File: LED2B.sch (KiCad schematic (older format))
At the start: 17 parts

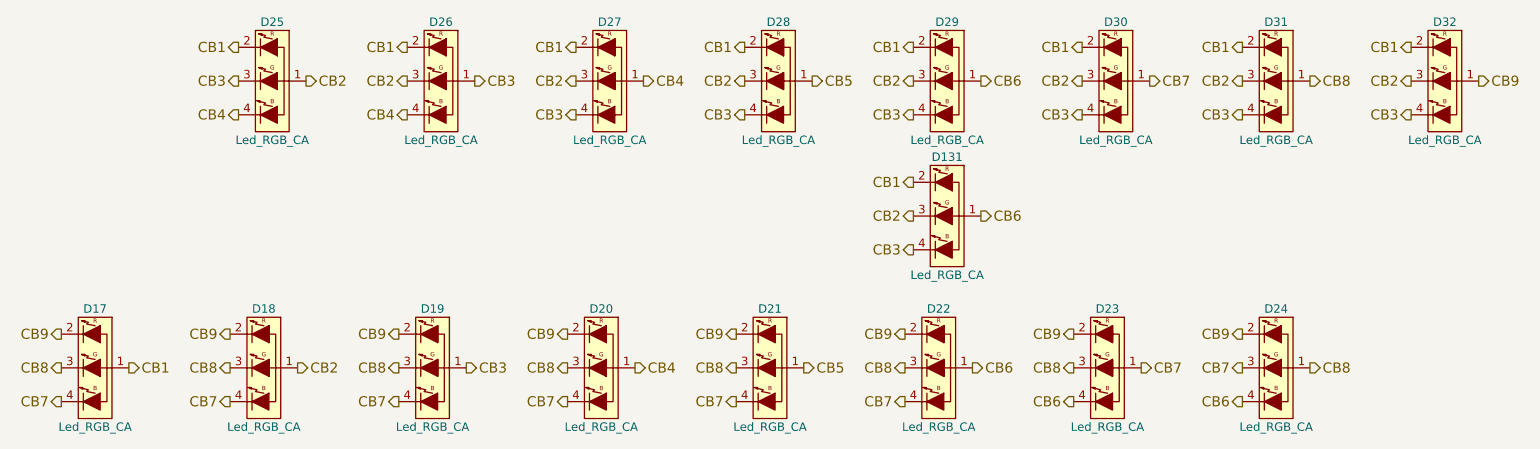
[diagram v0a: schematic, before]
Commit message: Did some visual cleanup.
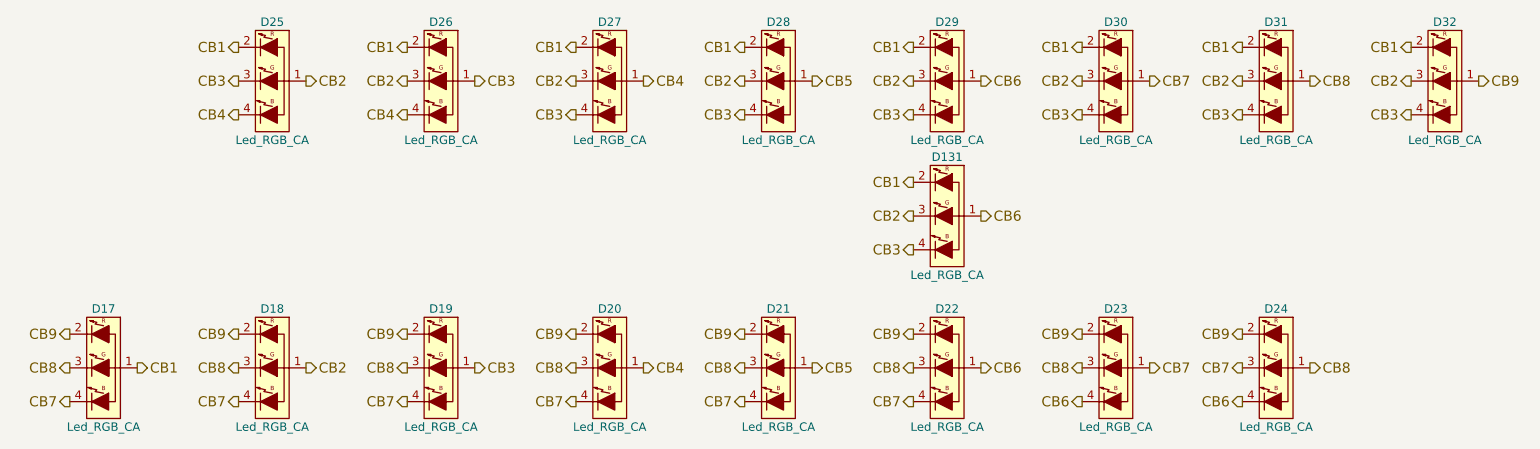
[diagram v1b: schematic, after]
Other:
- moved on the sheet: D17, D18, D19, D20, D21, D22, D23
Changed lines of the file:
@@
 $Descr A4 11693 8268
 encoding utf-8
-Sheet 3 6
+Sheet 2 6
 Title ""
 Date ""
@@
 Text HLabel 9750 1550 0    60   Output ~ 0
 CB1
-Text HLabel 2150 3450 2    60   Output ~ 0
-CB1
-Text HLabel 1750 3650 0    60   Output ~ 0
-CB7
-Text HLabel 1750 3450 0    60   Output ~ 0
-CB8
-Text HLabel 1750 3250 0    60   Output ~ 0
-CB9
-Text HLabel 2750 3650 0    60   Output ~ 0
-CB7
-Text HLabel 2750 3450 0    60   Output ~ 0
-CB8
-Text HLabel 2750 3250 0    60   Output ~ 0
-CB9
-Text HLabel 3150 3450 2    60   Output ~ 0
-CB2
-Text HLabel 3750 3650 0    60   Output ~ 0
-CB7
-Text HLabel 3750 3450 0    60   Output ~ 0
-CB8
-Text HLabel 3750 3250 0    60   Output ~ 0
-CB9
-Text HLabel 4150 3450 2    60   Output ~ 0
-CB3
-Text HLabel 4750 3650 0    60   Output ~ 0
-CB7
-Text HLabel 4750 3450 0    60   Output ~ 0
-CB8
-Text HLabel 4750 3250 0    60   Output ~ 0
-CB9
-Text HLabel 5150 3450 2    60   Output ~ 0
+Text HLabel 2200 3450 2    60   Output ~ 0
+CB1
+Text HLabel 1800 3650 0    60   Output ~ 0
+CB7
+Text HLabel 1800 3450 0    60   Output ~ 0
+CB8
+Text HLabel 1800 3250 0    60   Output ~ 0
+CB9
+Text HLabel 2800 3650 0    60   Output ~ 0
+CB7
+Text HLabel 2800 3450 0    60   Output ~ 0
+CB8
+Text HLabel 2800 3250 0    60   Output ~ 0
+CB9
+Text HLabel 3200 3450 2    60   Output ~ 0
+CB2
+Text HLabel 3800 3650 0    60   Output ~ 0
+CB7
+Text HLabel 3800 3450 0    60   Output ~ 0
+CB8
+Text HLabel 3800 3250 0    60   Output ~ 0
+CB9
+Text HLabel 4200 3450 2    60   Output ~ 0
+CB3
+Text HLabel 4800 3650 0    60   Output ~ 0
+CB7
+Text HLabel 4800 3450 0    60   Output ~ 0
+CB8
+Text HLabel 4800 3250 0    60   Output ~ 0
+CB9
+Text HLabel 5200 3450 2    60   Output ~ 0
 CB4
-Text HLabel 5750 3650 0    60   Output ~ 0
-CB7
-Text HLabel 5750 3450 0    60   Output ~ 0
-CB8
-Text HLabel 5750 3250 0    60   Output ~ 0
-CB9
-Text HLabel 6150 3450 2    60   Output ~ 0
+Text HLabel 5800 3650 0    60   Output ~ 0
+CB7
+Text HLabel 5800 3450 0    60   Output ~ 0
+CB8
+Text HLabel 5800 3250 0    60   Output ~ 0
+CB9
+Text HLabel 6200 3450 2    60   Output ~ 0
 CB5
-Text HLabel 6750 3650 0    60   Output ~ 0
-CB7
-Text HLabel 6750 3450 0    60   Output ~ 0
-CB8
-Text HLabel 6750 3250 0    60   Output ~ 0
-CB9
-Text HLabel 7150 3450 2    60   Output ~ 0
+Text HLabel 6800 3650 0    60   Output ~ 0
+CB7
+Text HLabel 6800 3450 0    60   Output ~ 0
+CB8
+Text HLabel 6800 3250 0    60   Output ~ 0
+CB9
+Text HLabel 7200 3450 2    60   Output ~ 0
 CB6
-Text HLabel 8150 3450 2    60   Output ~ 0
-CB7
-Text HLabel 7750 3450 0    60   Output ~ 0
-CB8
-Text HLabel 7750 3250 0    60   Output ~ 0
-CB9
-Text HLabel 7750 3650 0    60   Output ~ 0
+Text HLabel 8200 3450 2    60   Output ~ 0
+CB7
+Text HLabel 7800 3450 0    60   Output ~ 0
+CB8
+Text HLabel 7800 3250 0    60   Output ~ 0
+CB9
+Text HLabel 7800 3650 0    60   Output ~ 0
 CB6
 Text HLabel 8750 3250 0    60   Output ~ 0
@@
 L Led_RGB_CA D17
 U 1 1 56C5D501
-P 1950 3450
-F 0 "D17" H 1950 3800 50  0000 C CNN
-F 1 "Led_RGB_CA" H 1950 3100 50  0000 C CNN
-F 2 "mx2a:RGB" H 1905 3400 50  0001 C CNN
-F 3 "" H 1905 3400 50  0000 C CNN
-	1    1950 3450
+P 2000 3450
+F 0 "D17" H 2000 3800 50  0000 C CNN
+F 1 "Led_RGB_CA" H 2000 3100 50  0000 C CNN
+F 2 "mx2a:RGB" H 1955 3400 50  0001 C CNN
+F 3 "" H 1955 3400 50  0000 C CNN
+	1    2000 3450
 	1    0    0    -1
 $EndComp
@@
 L Led_RGB_CA D18
 U 1 1 56C5DE77
-P 2950 3450
-F 0 "D18" H 2950 3800 50  0000 C CNN
-F 1 "Led_RGB_CA" H 2950 3100 50  0000 C CNN
-F 2 "mx2a:RGB" H 2905 3400 50  0001 C CNN
-F 3 "" H 2905 3400 50  0000 C CNN
-	1    2950 3450
+P 3000 3450
+F 0 "D18" H 3000 3800 50  0000 C CNN
+F 1 "Led_RGB_CA" H 3000 3100 50  0000 C CNN
+F 2 "mx2a:RGB" H 2955 3400 50  0001 C CNN
+F 3 "" H 2955 3400 50  0000 C CNN
+	1    3000 3450
 	1    0    0    -1
 $EndComp
@@
 L Led_RGB_CA D19
 U 1 1 56C5DEC1
-P 3950 3450
-F 0 "D19" H 3950 3800 50  0000 C CNN
-F 1 "Led_RGB_CA" H 3950 3100 50  0000 C CNN
-F 2 "mx2a:RGB" H 3905 3400 50  0001 C CNN
-F 3 "" H 3905 3400 50  0000 C CNN
-	1    3950 3450
+P 4000 3450
+F 0 "D19" H 4000 3800 50  0000 C CNN
+F 1 "Led_RGB_CA" H 4000 3100 50  0000 C CNN
+F 2 "mx2a:RGB" H 3955 3400 50  0001 C CNN
+F 3 "" H 3955 3400 50  0000 C CNN
+	1    4000 3450
 	1    0    0    -1
 $EndComp
@@
 L Led_RGB_CA D20
 U 1 1 56C5DF12
-P 4950 3450
-F 0 "D20" H 4950 3800 50  0000 C CNN
-F 1 "Led_RGB_CA" H 4950 3100 50  0000 C CNN
-F 2 "mx2a:RGB" H 4905 3400 50  0001 C CNN
-F 3 "" H 4905 3400 50  0000 C CNN
-	1    4950 3450
+P 5000 3450
+F 0 "D20" H 5000 3800 50  0000 C CNN
+F 1 "Led_RGB_CA" H 5000 3100 50  0000 C CNN
+F 2 "mx2a:RGB" H 4955 3400 50  0001 C CNN
+F 3 "" H 4955 3400 50  0000 C CNN
+	1    5000 3450
 	1    0    0    -1
 $EndComp
@@
 L Led_RGB_CA D21
 U 1 1 56C5E004
-P 5950 3450
-F 0 "D21" H 5950 3800 50  0000 C CNN
-F 1 "Led_RGB_CA" H 5950 3100 50  0000 C CNN
-F 2 "mx2a:RGB" H 5905 3400 50  0001 C CNN
-F 3 "" H 5905 3400 50  0000 C CNN
-	1    5950 3450
+P 6000 3450
+F 0 "D21" H 6000 3800 50  0000 C CNN
+F 1 "Led_RGB_CA" H 6000 3100 50  0000 C CNN
+F 2 "mx2a:RGB" H 5955 3400 50  0001 C CNN
+F 3 "" H 5955 3400 50  0000 C CNN
+	1    6000 3450
 	1    0    0    -1
 $EndComp
@@
 L Led_RGB_CA D22
 U 1 1 56C5E0ED
-P 6950 3450
-F 0 "D22" H 6950 3800 50  0000 C CNN
-F 1 "Led_RGB_CA" H 6950 3100 50  0000 C CNN
-F 2 "mx2a:RGB" H 6905 3400 50  0001 C CNN
-F 3 "" H 6905 3400 50  0000 C CNN
-	1    6950 3450
+P 7000 3450
+F 0 "D22" H 7000 3800 50  0000 C CNN
+F 1 "Led_RGB_CA" H 7000 3100 50  0000 C CNN
+F 2 "mx2a:RGB" H 6955 3400 50  0001 C CNN
+F 3 "" H 6955 3400 50  0000 C CNN
+	1    7000 3450
 	1    0    0    -1
 $EndComp
@@
 L Led_RGB_CA D23
 U 1 1 56C5E285
-P 7950 3450
-F 0 "D23" H 7950 3800 50  0000 C CNN
-F 1 "Led_RGB_CA" H 7950 3100 50  0000 C CNN
-F 2 "mx2a:RGB" H 7905 3400 50  0001 C CNN
-F 3 "" H 7905 3400 50  0000 C CNN
-	1    7950 3450
-	1    0    0    -1
-$EndComp
+P 8000 3450
+F 0 "D23" H 8000 3800 50  0000 C CNN
+F 1 "Led_RGB_CA" H 8000 3100 50  0000 C CNN
+F 2 "mx2a:RGB" H 7955 3400 50  0001 C CNN
+F 3 "" H 7955 3400 50  0000 C CNN
+	1    8000 3450
+	1    0    0    -1
+$EndComp

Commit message: Switched to a different USB Port and 100uF Cap
also added a USB-Debug Header and did some cleanup
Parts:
- D131, D17, D18, D19, D20, D21, D22, D23, D24, D25, D26, D27, D28, D29, D30, D31, D32: footprint mx2a:RGB -> libs.pretty:RGB
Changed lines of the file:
@@
 U 1 1 56C58153
 P 3000 1750
+AR Path="/56C58153" Ref="D25"  Part="1"
+AR Path="/572AC680/56C58153" Ref="D25"  Part="1"
 F 0 "D25" H 3000 2100 50  0000 C CNN
 F 1 "Led_RGB_CA" H 3000 1400 50  0000 C CNN
-F 2 "mx2a:RGB" H 2955 1700 50  0001 C CNN
+F 2 "libs.pretty:RGB" H 2955 1700 50  0001 C CNN
 F 3 "" H 2955 1700 50  0000 C CNN
 	1    3000 1750
@@
 U 1 1 56C58187
 P 4000 1750
+AR Path="/56C58187" Ref="D26"  Part="1"
+AR Path="/572AC680/56C58187" Ref="D26"  Part="1"
 F 0 "D26" H 4000 2100 50  0000 C CNN
 F 1 "Led_RGB_CA" H 4000 1400 50  0000 C CNN
-F 2 "mx2a:RGB" H 3955 1700 50  0001 C CNN
+F 2 "libs.pretty:RGB" H 3955 1700 50  0001 C CNN
 F 3 "" H 3955 1700 50  0000 C CNN
 	1    4000 1750
@@
 U 1 1 56C581B9
 P 5000 1750
+AR Path="/56C581B9" Ref="D27"  Part="1"
+AR Path="/572AC680/56C581B9" Ref="D27"  Part="1"
 F 0 "D27" H 5000 2100 50  0000 C CNN
 F 1 "Led_RGB_CA" H 5000 1400 50  0000 C CNN
-F 2 "mx2a:RGB" H 4955 1700 50  0001 C CNN
+F 2 "libs.pretty:RGB" H 4955 1700 50  0001 C CNN
 F 3 "" H 4955 1700 50  0000 C CNN
 	1    5000 1750
@@
 U 1 1 56C5823E
 P 6000 1750
+AR Path="/56C5823E" Ref="D28"  Part="1"
+AR Path="/572AC680/56C5823E" Ref="D28"  Part="1"
 F 0 "D28" H 6000 2100 50  0000 C CNN
 F 1 "Led_RGB_CA" H 6000 1400 50  0000 C CNN
-F 2 "mx2a:RGB" H 5955 1700 50  0001 C CNN
+F 2 "libs.pretty:RGB" H 5955 1700 50  0001 C CNN
 F 3 "" H 5955 1700 50  0000 C CNN
 	1    6000 1750
@@
 U 1 1 56C582F6
 P 7000 1750
+AR Path="/56C582F6" Ref="D29"  Part="1"
+AR Path="/572AC680/56C582F6" Ref="D29"  Part="1"
 F 0 "D29" H 7000 2100 50  0000 C CNN
 F 1 "Led_RGB_CA" H 7000 1400 50  0000 C CNN
-F 2 "mx2a:RGB" H 6955 1700 50  0001 C CNN
+F 2 "libs.pretty:RGB" H 6955 1700 50  0001 C CNN
 F 3 "" H 6955 1700 50  0000 C CNN
 	1    7000 1750
@@
 U 1 1 56C58401
 P 8000 1750
+AR Path="/56C58401" Ref="D30"  Part="1"
+AR Path="/572AC680/56C58401" Ref="D30"  Part="1"
 F 0 "D30" H 8000 2100 50  0000 C CNN
 F 1 "Led_RGB_CA" H 8000 1400 50  0000 C CNN
-F 2 "mx2a:RGB" H 7955 1700 50  0001 C CNN
+F 2 "libs.pretty:RGB" H 7955 1700 50  0001 C CNN
 F 3 "" H 7955 1700 50  0000 C CNN
 	1    8000 1750
@@
 U 1 1 56C584BD
 P 8950 1750
+AR Path="/56C584BD" Ref="D31"  Part="1"
+AR Path="/572AC680/56C584BD" Ref="D31"  Part="1"
 F 0 "D31" H 8950 2100 50  0000 C CNN
 F 1 "Led_RGB_CA" H 8950 1400 50  0000 C CNN
-F 2 "mx2a:RGB" H 8905 1700 50  0001 C CNN
+F 2 "libs.pretty:RGB" H 8905 1700 50  0001 C CNN
 F 3 "" H 8905 1700 50  0000 C CNN
 	1    8950 1750
@@
 U 1 1 56C5CB8C
 P 9950 1750
+AR Path="/56C5CB8C" Ref="D32"  Part="1"
+AR Path="/572AC680/56C5CB8C" Ref="D32"  Part="1"
 F 0 "D32" H 9950 2100 50  0000 C CNN
 F 1 "Led_RGB_CA" H 9950 1400 50  0000 C CNN
-F 2 "mx2a:RGB" H 9905 1700 50  0001 C CNN
+F 2 "libs.pretty:RGB" H 9905 1700 50  0001 C CNN
 F 3 "" H 9905 1700 50  0000 C CNN
 	1    9950 1750
@@
 U 1 1 56C5D501
 P 2000 3450
+AR Path="/56C5D501" Ref="D17"  Part="1"
+AR Path="/572AC680/56C5D501" Ref="D17"  Part="1"
 F 0 "D17" H 2000 3800 50  0000 C CNN
 F 1 "Led_RGB_CA" H 2000 3100 50  0000 C CNN
-F 2 "mx2a:RGB" H 1955 3400 50  0001 C CNN
+F 2 "libs.pretty:RGB" H 1955 3400 50  0001 C CNN
 F 3 "" H 1955 3400 50  0000 C CNN
 	1    2000 3450
@@
 U 1 1 56C5DE77
 P 3000 3450
+AR Path="/56C5DE77" Ref="D18"  Part="1"
+AR Path="/572AC680/56C5DE77" Ref="D18"  Part="1"
 F 0 "D18" H 3000 3800 50  0000 C CNN
 F 1 "Led_RGB_CA" H 3000 3100 50  0000 C CNN
-F 2 "mx2a:RGB" H 2955 3400 50  0001 C CNN
+F 2 "libs.pretty:RGB" H 2955 3400 50  0001 C CNN
 F 3 "" H 2955 3400 50  0000 C CNN
 	1    3000 3450
@@
 U 1 1 56C5DEC1
 P 4000 3450
+AR Path="/56C5DEC1" Ref="D19"  Part="1"
+AR Path="/572AC680/56C5DEC1" Ref="D19"  Part="1"
 F 0 "D19" H 4000 3800 50  0000 C CNN
 F 1 "Led_RGB_CA" H 4000 3100 50  0000 C CNN
-F 2 "mx2a:RGB" H 3955 3400 50  0001 C CNN
+F 2 "libs.pretty:RGB" H 3955 3400 50  0001 C CNN
 F 3 "" H 3955 3400 50  0000 C CNN
 	1    4000 3450
@@
 U 1 1 56C5DF12
 P 5000 3450
+AR Path="/56C5DF12" Ref="D20"  Part="1"
+AR Path="/572AC680/56C5DF12" Ref="D20"  Part="1"
 F 0 "D20" H 5000 3800 50  0000 C CNN
 F 1 "Led_RGB_CA" H 5000 3100 50  0000 C CNN
-F 2 "mx2a:RGB" H 4955 3400 50  0001 C CNN
+F 2 "libs.pretty:RGB" H 4955 3400 50  0001 C CNN
 F 3 "" H 4955 3400 50  0000 C CNN
 	1    5000 3450
@@
 U 1 1 56C5E004
 P 6000 3450
+AR Path="/56C5E004" Ref="D21"  Part="1"
+AR Path="/572AC680/56C5E004" Ref="D21"  Part="1"
 F 0 "D21" H 6000 3800 50  0000 C CNN
 F 1 "Led_RGB_CA" H 6000 3100 50  0000 C CNN
-F 2 "mx2a:RGB" H 5955 3400 50  0001 C CNN
+F 2 "libs.pretty:RGB" H 5955 3400 50  0001 C CNN
 F 3 "" H 5955 3400 50  0000 C CNN
 	1    6000 3450
@@
 U 1 1 56C5E0ED
 P 7000 3450
+AR Path="/56C5E0ED" Ref="D22"  Part="1"
+AR Path="/572AC680/56C5E0ED" Ref="D22"  Part="1"
 F 0 "D22" H 7000 3800 50  0000 C CNN
 F 1 "Led_RGB_CA" H 7000 3100 50  0000 C CNN
-F 2 "mx2a:RGB" H 6955 3400 50  0001 C CNN
+F 2 "libs.pretty:RGB" H 6955 3400 50  0001 C CNN
 F 3 "" H 6955 3400 50  0000 C CNN
 	1    7000 3450
@@
 U 1 1 56C5E285
 P 8000 3450
+AR Path="/56C5E285" Ref="D23"  Part="1"
+AR Path="/572AC680/56C5E285" Ref="D23"  Part="1"
 F 0 "D23" H 8000 3800 50  0000 C CNN
 F 1 "Led_RGB_CA" H 8000 3100 50  0000 C CNN
-F 2 "mx2a:RGB" H 7955 3400 50  0001 C CNN
+F 2 "libs.pretty:RGB" H 7955 3400 50  0001 C CNN
 F 3 "" H 7955 3400 50  0000 C CNN
 	1    8000 3450
@@
 U 1 1 56C5E3D6
 P 8950 3450
+AR Path="/56C5E3D6" Ref="D24"  Part="1"
+AR Path="/572AC680/56C5E3D6" Ref="D24"  Part="1"
 F 0 "D24" H 8950 3800 50  0000 C CNN
 F 1 "Led_RGB_CA" H 8950 3100 50  0000 C CNN
-F 2 "mx2a:RGB" H 8905 3400 50  0001 C CNN
+F 2 "libs.pretty:RGB" H 8905 3400 50  0001 C CNN
 F 3 "" H 8905 3400 50  0000 C CNN
 	1    8950 3450
@@
 U 1 1 56EDA7FD
 P 7000 2550
+AR Path="/56EDA7FD" Ref="D131"  Part="1"
+AR Path="/572AC680/56EDA7FD" Ref="D131"  Part="1"
 F 0 "D131" H 7000 2900 50  0000 C CNN
 F 1 "Led_RGB_CA" H 7000 2200 50  0000 C CNN
-F 2 "mx2a:RGB" H 6955 2500 50  0001 C CNN
+F 2 "libs.pretty:RGB" H 6955 2500 50  0001 C CNN
 F 3 "" H 6955 2500 50  0000 C CNN
 	1    7000 2550
